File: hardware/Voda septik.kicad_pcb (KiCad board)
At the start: 2 copper layers, 67.7 x 86.4 mm, 41 parts, among them J1 Napájení a 4-20mA senzory, J2 Screw_Terminal_01x09, J3 Display LCD I2C, J4 Display TM1637, U1 DC-DC 24V -> 5V, U2 MAX3485-modul, U3 ADS1115IDGS, U4 ESP32-DevKitC, U5 CA56-12CGKWA

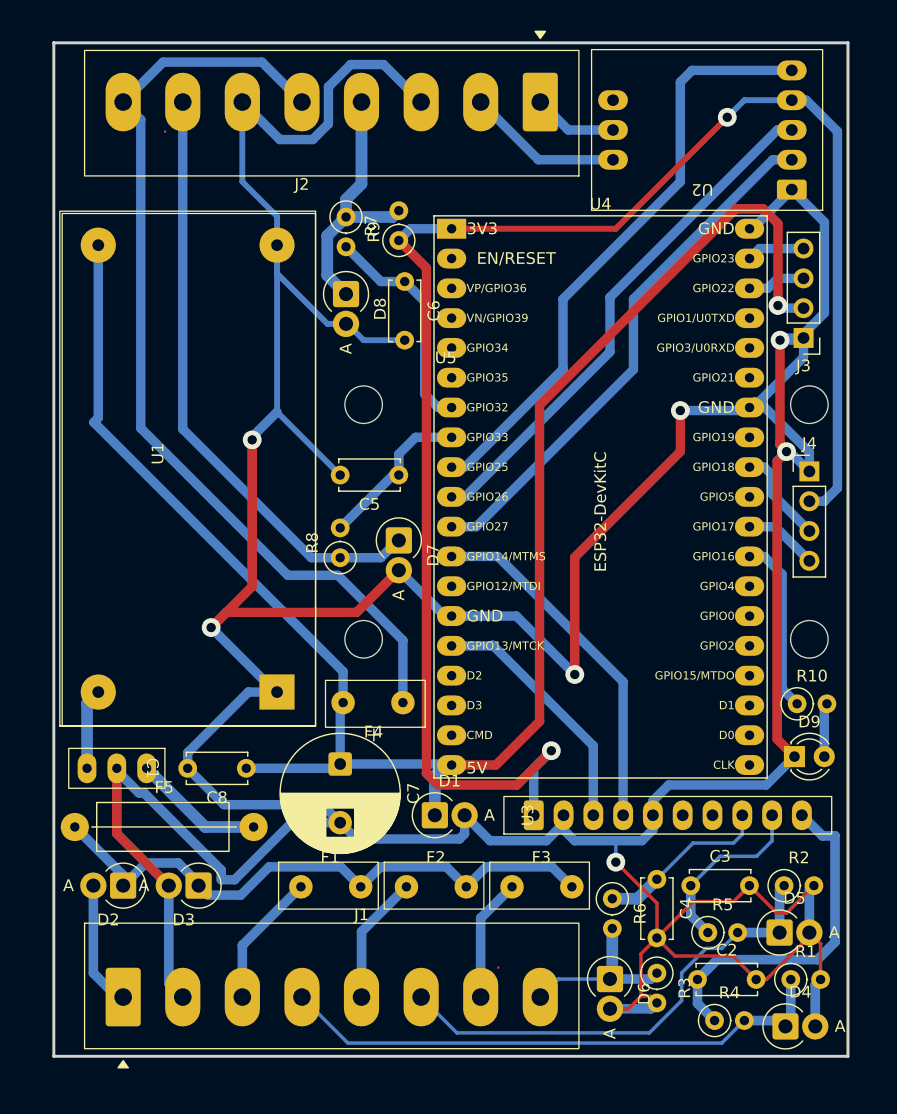
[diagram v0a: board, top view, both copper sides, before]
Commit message: Hotový návrh desky a schématu, které jdou do výroby.
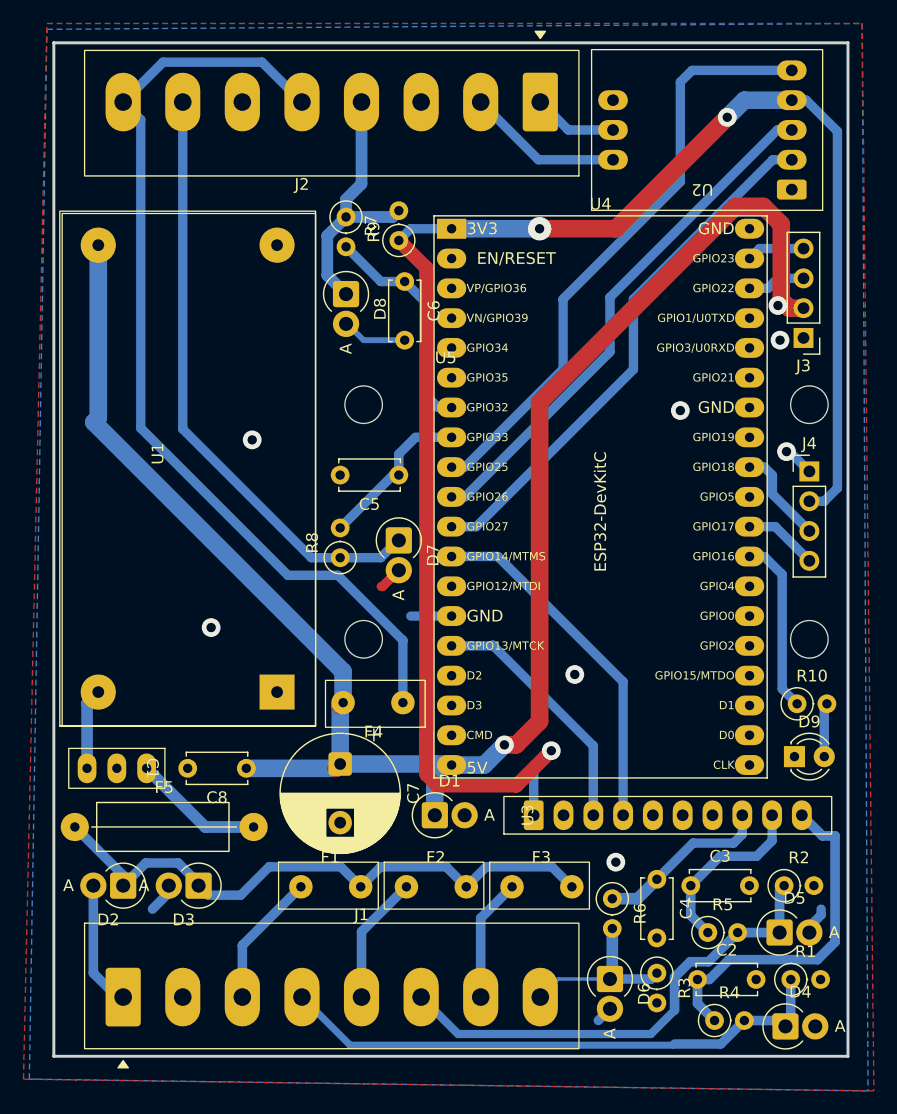
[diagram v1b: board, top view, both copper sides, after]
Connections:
- U4 pad 16: (no net) -> unconnected-(U4-SD_DATA2/GPIO9-Pad16)
- U4 pad 17: (no net) -> unconnected-(U4-SD_DATA3/GPIO10-Pad17)
- U4 pad 18: (no net) -> unconnected-(U4-CMD-Pad18)
- U4 pad 20: (no net) -> unconnected-(U4-SD_CLK/GPIO6-Pad20)
- U4 pad 21: (no net) -> unconnected-(U4-SD_DATA0/GPIO7-Pad21)
- U4 pad 22: (no net) -> unconnected-(U4-SD_DATA1/GPIO8-Pad22)
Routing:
- net GND: track 444.0 -> 20.6 mm
- net +3.3V: track 141.5 -> 157.3 mm, vias 2 -> 3
- net +5V: track 149.2 -> 151.6 mm, vias 1 -> 2
- added copper zone on B.Cu, net GND
- added copper zone on F.Cu, net GND
